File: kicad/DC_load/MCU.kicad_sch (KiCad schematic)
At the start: 132 parts, among them J1 BNC, J10 DC fan connector, J6 USB_B, J8 FT232 programming port, J9 Conn_01x04_Socket, Q1 MMBT5401, Q13 AO3400A, SW1 RotaryEncoder_Switch, SW2 RotaryEncoder_Switch, SW3 SW_Push, SW8 SW_Push, U1 FSA3157P6X, U10 FSA3157P6X, U11 FSA3157P6X, U12 FSA3157P6X, U14 AMS1117-3.3, U15 74HC14D653, U16 93LCxxB, U17 CH340C, U18 TL431DBZ, U2 Screen, U8 STM32F103C8Tx

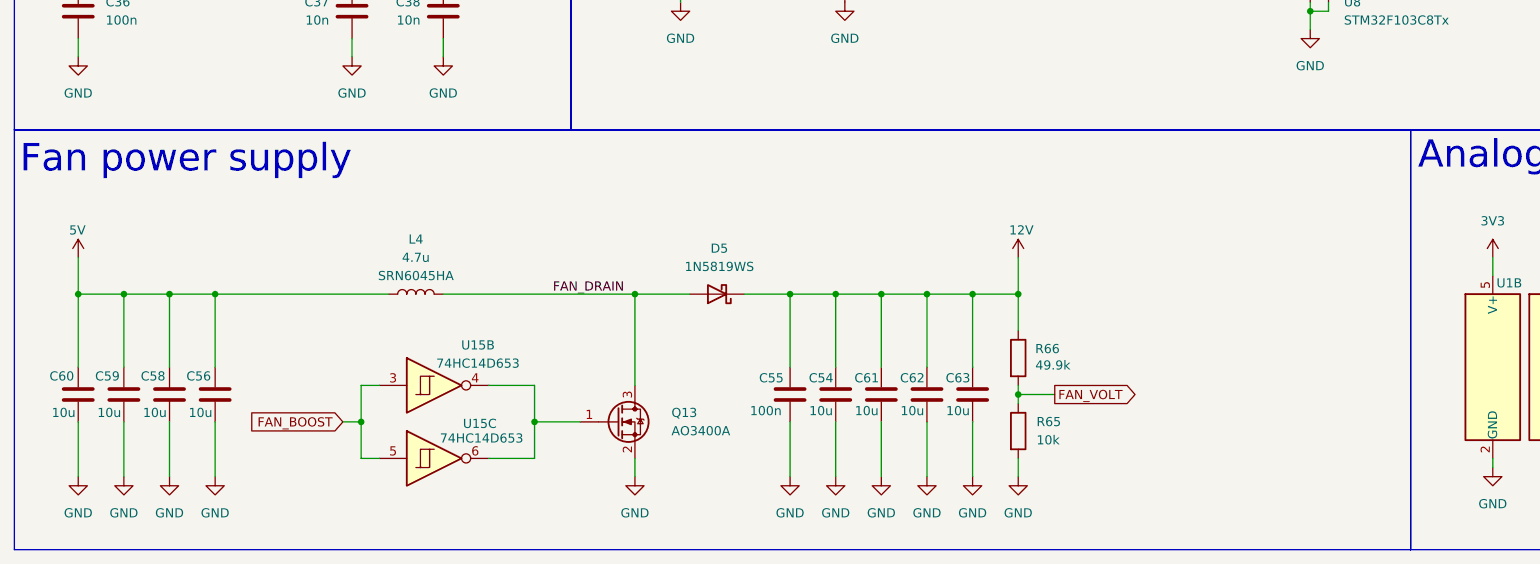
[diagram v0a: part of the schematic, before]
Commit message: Sim, comp, power.
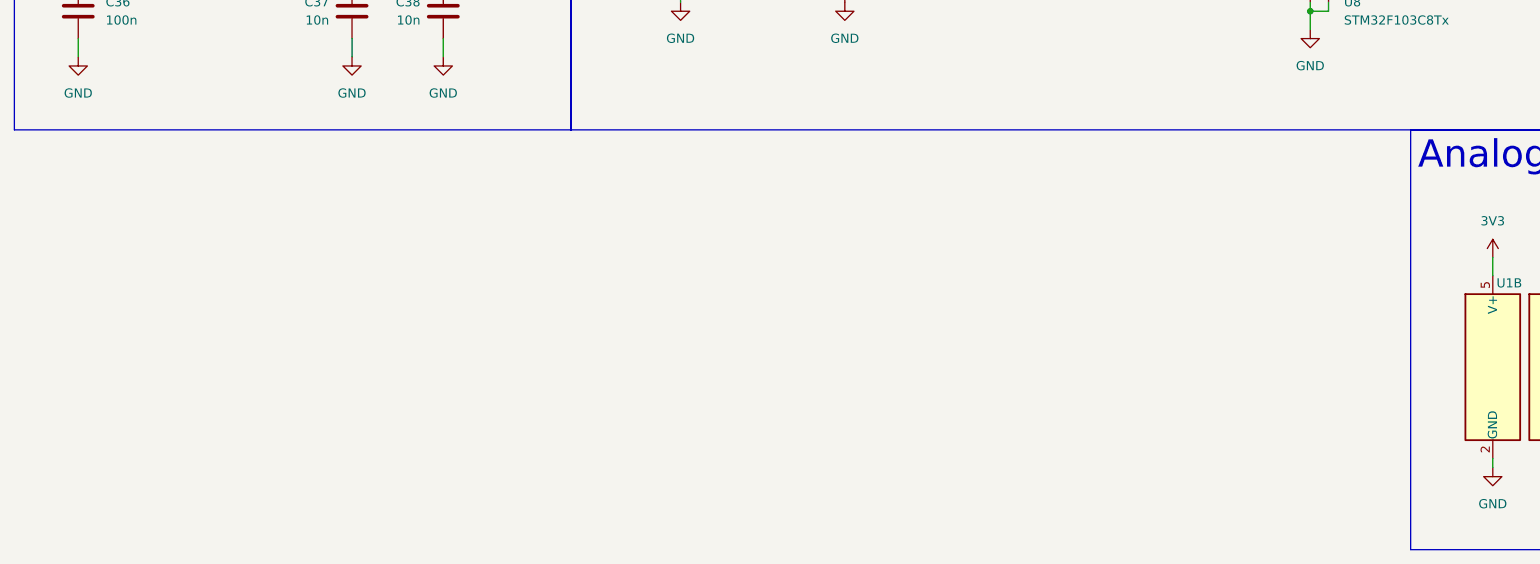
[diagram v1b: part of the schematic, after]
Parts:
- removed C54, C56, C58, C59, C60, C61, C62, C63: 10u, Capacitor_SMD:C_0603_1608Metric_Pad1.08x0.95mm_HandSolder, symbol Device:C
- removed C55: 100n, Capacitor_SMD:C_0603_1608Metric_Pad1.08x0.95mm_HandSolder, symbol Device:C
- removed D5: 1N5819WS, Diode_SMD:D_SOD-323, symbol Diode:1N5819WS
- removed L4: 4.7u, DC_load:L_Bourns_SRN6045TA, symbol solar_push_pull_sym_lib:SRN6045HA-4R7Y
- removed Q13: AO3400A, Package_TO_SOT_SMD:SOT-23, symbol Transistor_FET:AO3400A
- removed R65: 10k, Resistor_SMD:R_0603_1608Metric_Pad0.98x0.95mm_HandSolder, symbol Device:R
- removed R66: 49.9k, Resistor_SMD:R_0603_1608Metric_Pad0.98x0.95mm_HandSolder, symbol Device:R
- removed unit 2 of U15
- removed unit 3 of U15
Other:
- note removed: "Fan power supply"
